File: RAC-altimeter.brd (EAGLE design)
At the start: 30.5 x 50.8 mm, 37 parts, among them J1 282834-2, J2 CORTEX_DEBUG_SMD, J3 JUMPER-SMT_2_NO_SILK, U1 MAX32660GTP+, U2 BMI088, U3 BMP388, U4 RN4871-I_RM130, U5 W25N01GVZEIG_TR, U6 MCP1640T-I_CHY, Y1 32.768kHz

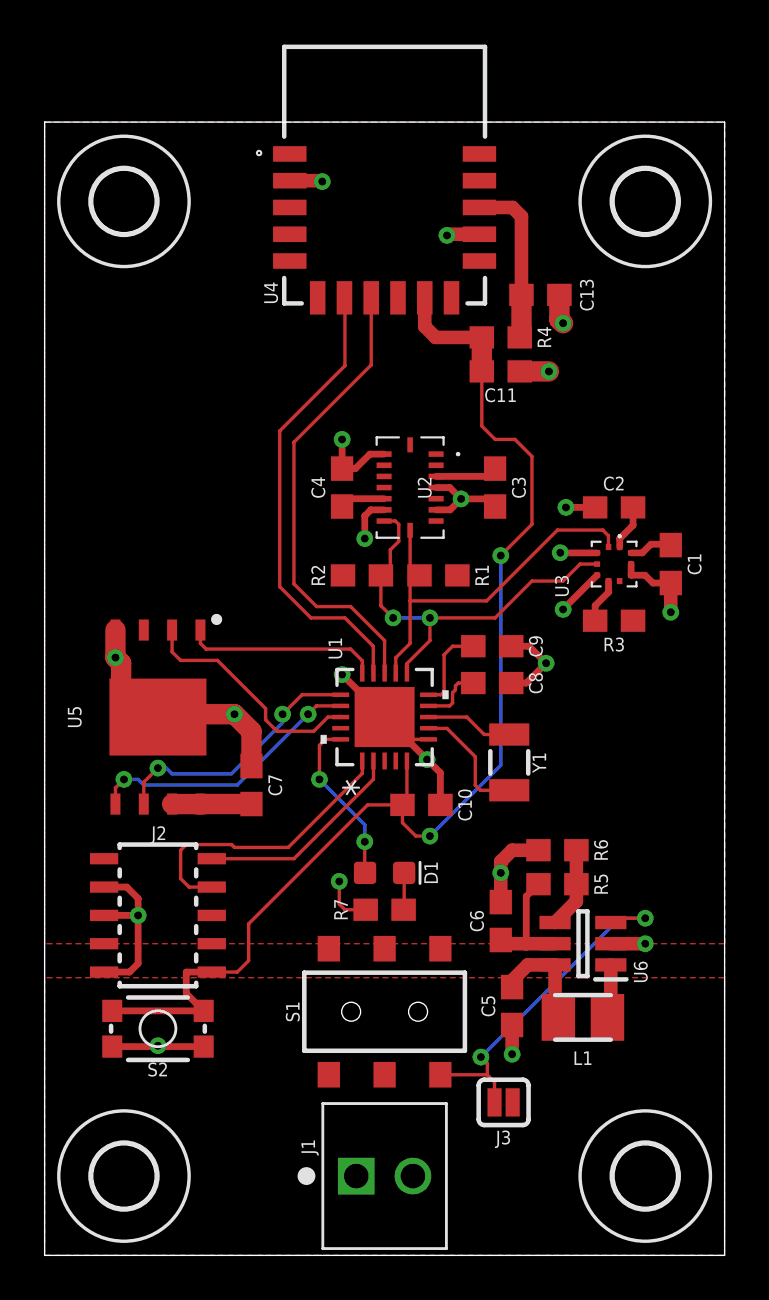
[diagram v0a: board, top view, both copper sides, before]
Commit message: Laid out parts neatly, routed board, removed unnecessary parts
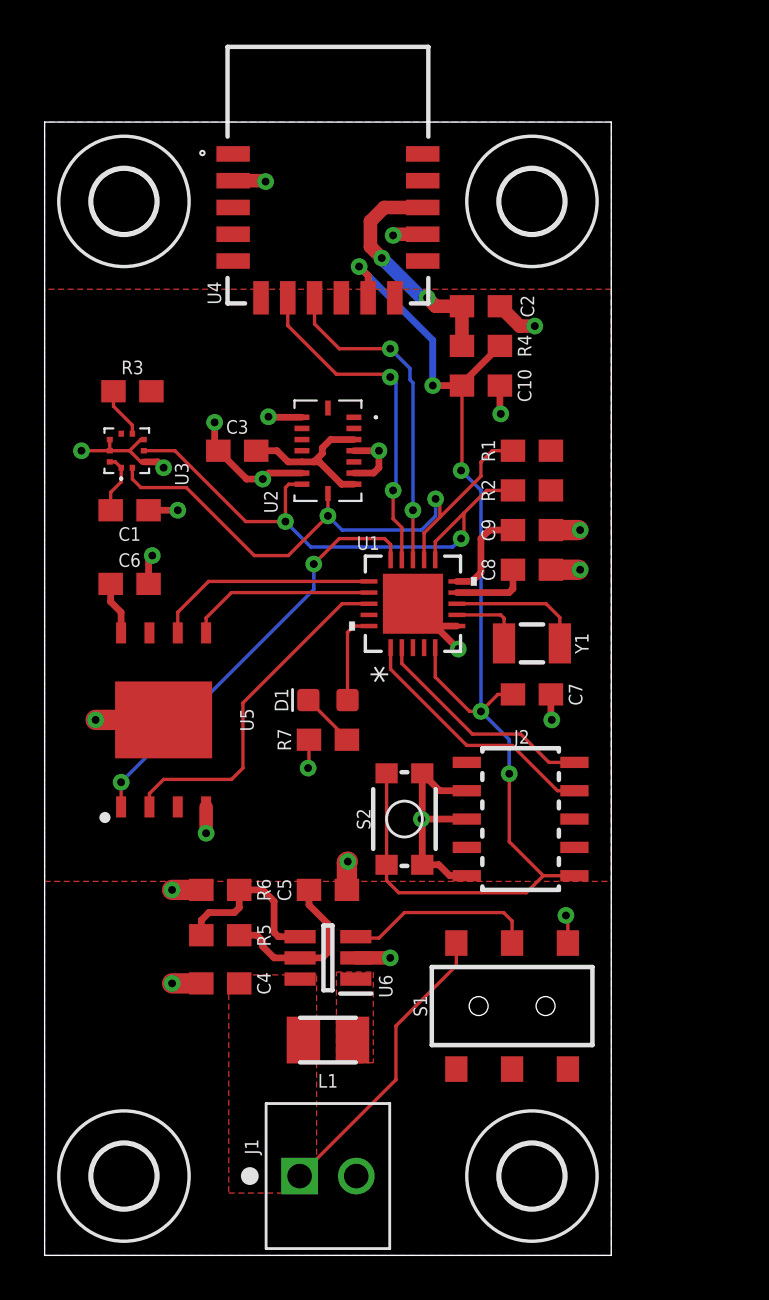
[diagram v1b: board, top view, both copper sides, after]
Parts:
- removed C11: 1.0uF, SparkFun-Capacitors:0603
- removed C13: 10uF, SparkFun-Capacitors:0603
- removed J3: JUMPER-SMT_2_NO_SILK, SparkFun-Jumpers:SMT-JUMPER_2_NO_SILK
- C10: value 0.1uF -> 1.0uF
- C2, C4: value 0.1uF -> 10uF
- C7: value 10uF -> 0.1uF
- moved C1 24.4 mm to (3.81, 33.4), turned to 0 degrees
- moved R3 23.9 mm to (3.94, 38.7)
- moved C4 22.9 mm to (7.87, 12.2), turned to 180 degrees
- moved C6 22.5 mm to (3.81, 30.1), turned to 0 degrees
- moved U3 22.4 mm to (3.68, 36.1), turned to 180 degrees
- moved C10 19.0 mm to (19.6, 39.0)
- moved J2 16.8 mm to (21.3, 19.6)
- moved R5 15.3 mm to (7.87, 14.4), turned to 0 degrees
- moved R6 15.2 mm to (7.87, 16.4)
- moved S2 14.5 mm to (16.1, 19.6), turned to 270 degrees
- moved C7 13.2 mm to (21.8, 25.1), turned to 0 degrees
- moved C3 11.7 mm to (8.64, 36.1), turned to 180 degrees
- moved L1 11.5 mm to (12.7, 9.65)
- moved U6 11.4 mm to (12.7, 13.3)
- moved C2 10.8 mm to (19.6, 42.5), turned to 0 degrees
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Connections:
- net !RSTN: now also C7.1; no longer C11.1
- net BOOST_EN: now also S1.2; no longer J3.2, S1.1
- net GND: now also C4.2, S1.3; no longer C11.2, C13.2, C4.1
- net VCC: now also C5.1; no longer C13.1, C4.2, C7.1
- net V_BATT: now also C4.1, S1.1; no longer C5.1, J3.1, S1.2
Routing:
- net GND: track 70.4 -> 56.5 mm, vias 22 -> 25
- net !SPI0_CS: track 8.73 -> 19.2 mm, vias 0 -> 2
- net I2C0_SCL: track 17.8 -> 26.5 mm, vias 0 -> 2
- net V_BATT: track 4.92 -> 13.4 mm
- net BOOST_EN: track 16.0 -> 8.65 mm, vias 2 -> 0
- net VCC: track 28.1 -> 34.4 mm, vias 0 -> 2
- net I2C0_SDA: track 18.6 -> 24.9 mm
- net UART1_RX: track 20.8 -> 14.9 mm, vias 0 -> 2
- net UART1_TX: track 20.7 -> 15.3 mm, vias 0 -> 2
- net SPI0_MISO: track 10.6 -> 15.7 mm
- net VFB: track 3.64 -> 7.82 mm
- net SPI0_MOSI: track 12.6 -> 8.44 mm, vias 2 -> 0
- net IO_LED: track 7.63 -> 4.12 mm, vias 2 -> 0
- net SW: track 2.41 -> 0.00 mm
- net 32KOUT: track 5.52 -> 3.30 mm
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- added copper zone on layer 1, net SW
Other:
- board size 30.5 x 50.8 mm -> 25.4 x 50.8 mm
